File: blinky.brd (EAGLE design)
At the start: 103.2 x 40 mm, 10 parts, among them IC1 LM555D, J1 1X2-3.5MM

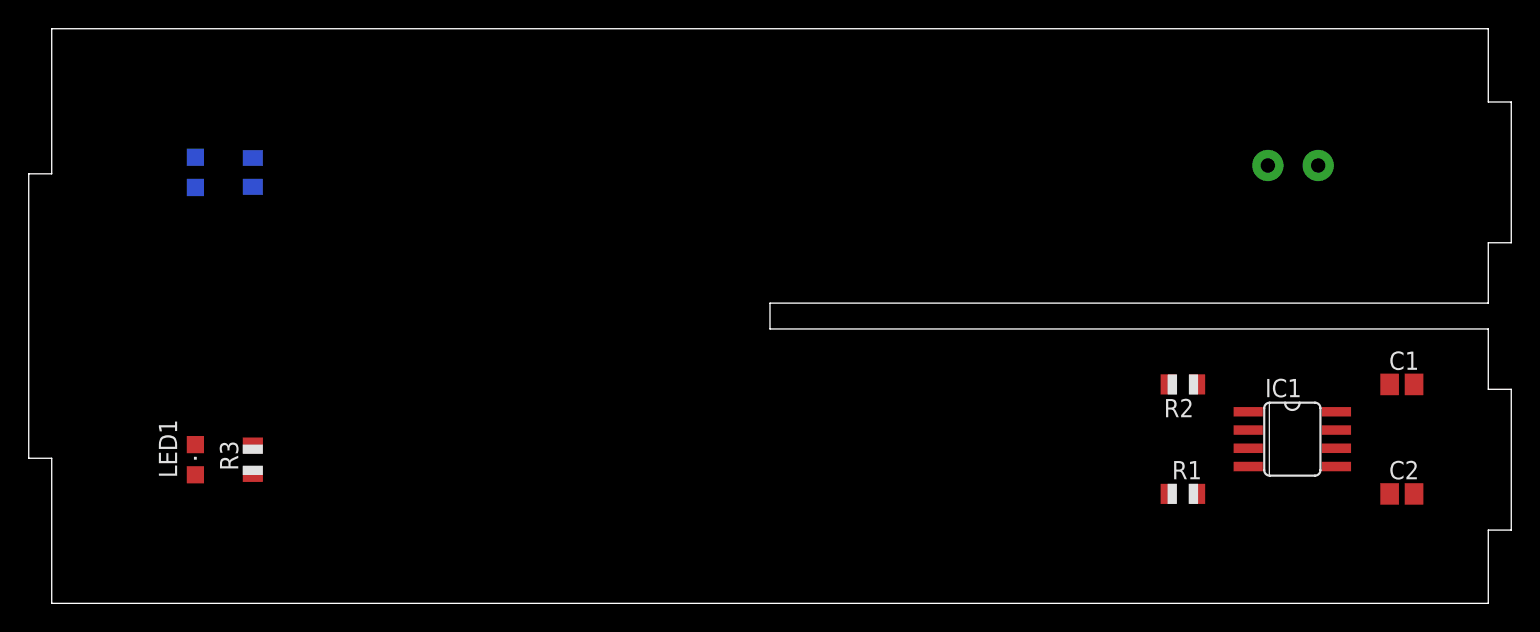
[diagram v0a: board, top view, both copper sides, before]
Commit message: eagle updated the file
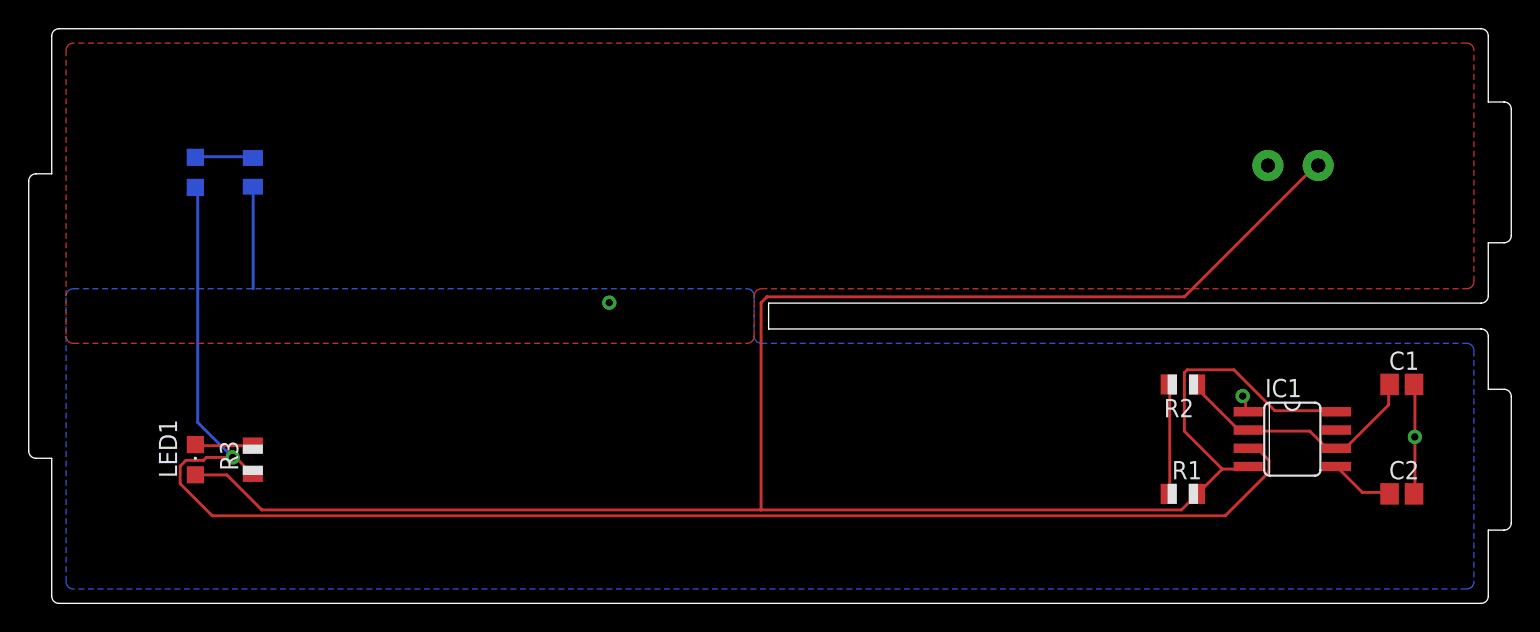
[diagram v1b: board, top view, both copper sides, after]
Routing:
- net VCC: track 0.00 -> 152.4 mm
- net N$2: track 0.00 -> 107.5 mm, vias 0 -> 1
- net N$6: track 0.00 -> 18.2 mm
- net GND: track 0.00 -> 16.1 mm, vias 0 -> 3
- net N$4: track 0.00 -> 7.74 mm
- net N$7: track 0.00 -> 4.50 mm
- net N$3: track 0.00 -> 4.03 mm
- net N$1: track 0.00 -> 4.02 mm
- added copper zone on layer 1, net GND
- added copper zone on layer 16, net GND
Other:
- outline, holes or cut-outs redrawn
